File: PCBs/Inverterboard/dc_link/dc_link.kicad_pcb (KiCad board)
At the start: 2 copper layers, 200 x 100.3 mm, 78 parts, among them J2 Conn_02x02_Odd_Even, J3 Conn_02x02_Odd_Even, J4 Conn_02x02_Odd_Even, J5 Conn_02x04_Odd_Even

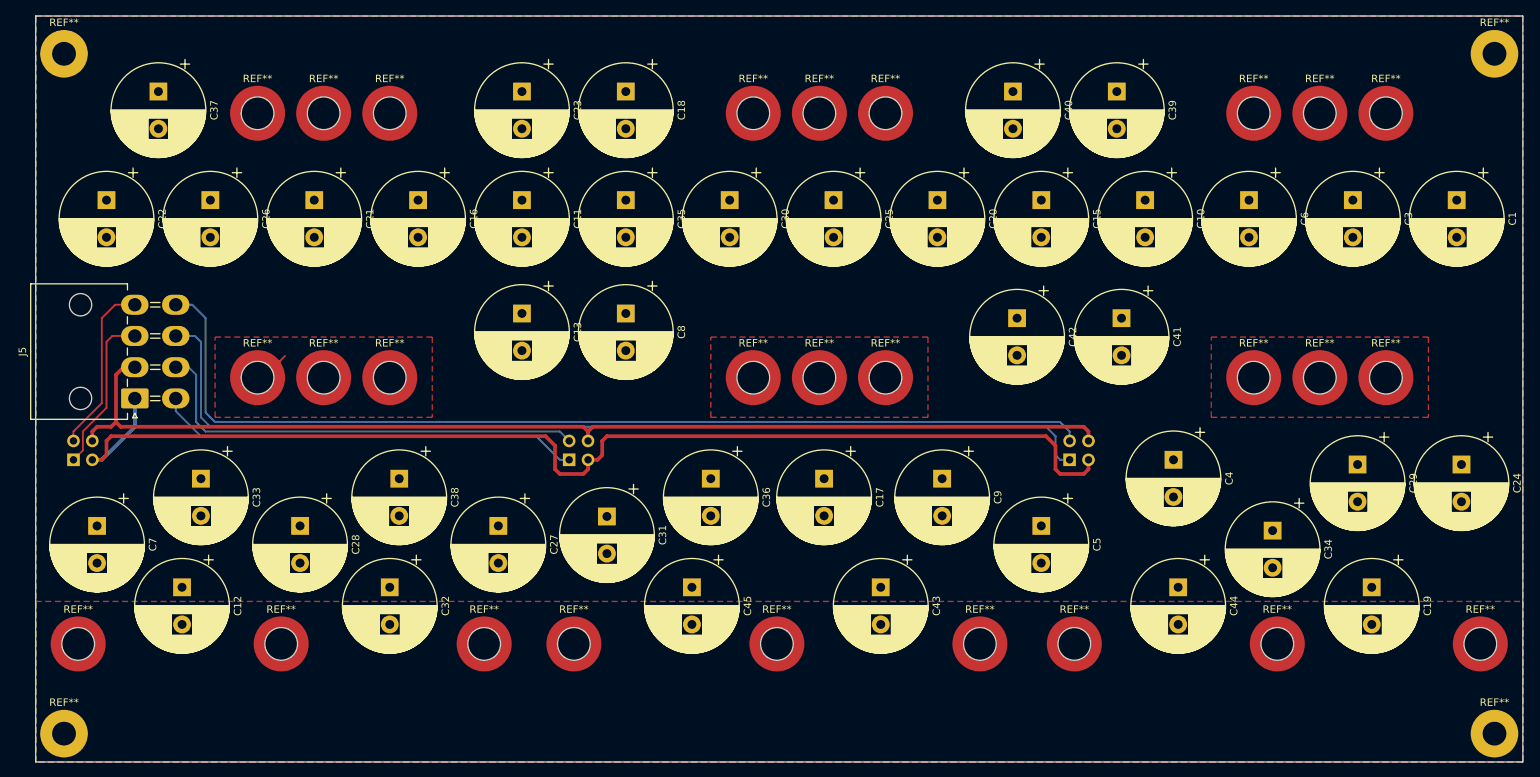
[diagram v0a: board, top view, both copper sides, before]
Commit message: Last fixes after PCB review
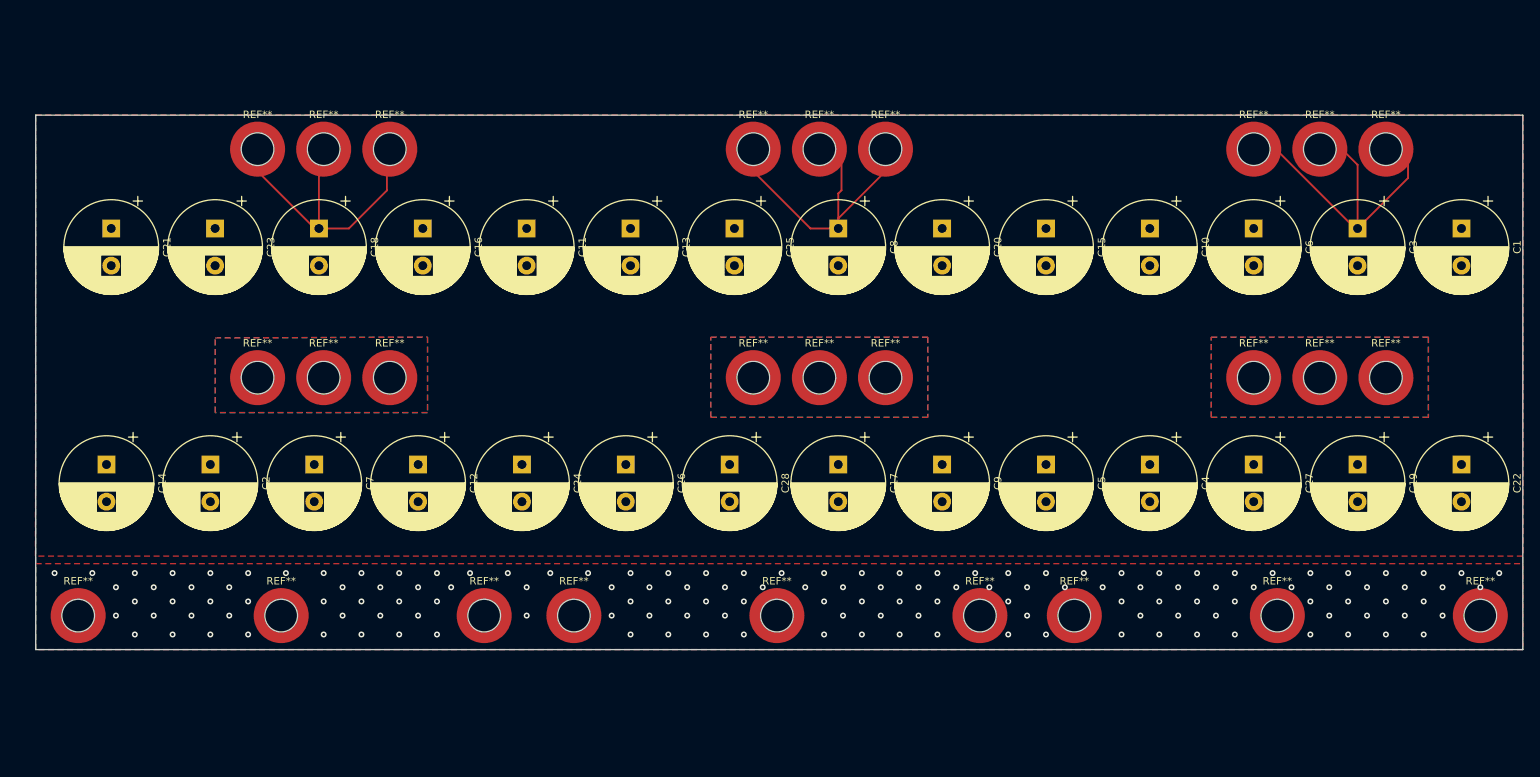
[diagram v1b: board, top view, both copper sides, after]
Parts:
- removed the C21 at (76.8, 62.9)
- removed the C23 at (104.8, 48.3)
- removed the C25 at (146.7, 62.9)
- removed the C27 at (101.6, 106.7)
- removed the C28 at (74.9, 106.7)
- removed C29, C31, C33, C35, C37, C38, C39, C40, C43, C44, C45: CP, Capacitor_THT:CP_Radial_D12.5mm_P5.00mm
- removed J2, J3, J4: Conn_02x02_Odd_Even, Connector_PinSocket_2.54mm:PinSocket_2x02_P2.54mm_Vertical
- removed J5: Conn_02x04_Odd_Even, Connector_Molex:Molex_Mini-Fit_Jr_5569-08A2_2x04_P4.20mm_Horizontal
- removed the REF** at (69.2, 51.2)
- removed the REF** at (45.1, 122.6)
- removed the REF** at (72.4, 122.6)
- removed the REF** at (78.1, 51.2)
- removed the REF** at (99.7, 122.6)
- removed the REF** at (111.8, 122.6)
- removed the REF** at (139.1, 122.6)
- removed the REF** at (166.4, 122.6)
- removed the REF** at (179.1, 122.6)
- removed the REF** at (206.4, 122.6)
- removed the REF** at (233.7, 122.6)
- removed the REF** at (43.2, 43.2)
- removed the REF** at (235.6, 43.2)
- removed the REF** at (235.6, 134.6)
- removed the REF** at (87.0, 51.2)
- removed the REF** at (43.2, 134.6)
- removed the REF** at (221.0, 51.2)
- removed the REF** at (135.9, 51.2)
- removed the REF** at (144.8, 51.2)
- removed the REF** at (153.7, 51.2)
- removed the REF** at (203.2, 51.2)
- removed the REF** at (212.1, 51.2)
- added C24: CP, Capacitor_THT:CP_Radial_D12.5mm_P5.00mm, F.Cu at (104.8, 98.4)
- added REF**: Mounting_Wuerth_WA-SMSR-M3_H2.6mm_ReverseMount_9775026360, Mounting_Wuerth:Mounting_Wuerth_WA-SMSR-M3_H2.6mm_ReverseMount_9775026360, F.Cu at (233.7, 118.7)
- added REF**: Mounting_Wuerth_WA-SMSR-M3_H2.6mm_ReverseMount_9775026360, Mounting_Wuerth:Mounting_Wuerth_WA-SMSR-M3_H2.6mm_ReverseMount_9775026360, F.Cu at (212.1, 56.0)
- added REF**: Mounting_Wuerth_WA-SMSR-M3_H2.6mm_ReverseMount_9775026360, Mounting_Wuerth:Mounting_Wuerth_WA-SMSR-M3_H2.6mm_ReverseMount_9775026360, F.Cu at (203.2, 56.0)
- added REF**: Mounting_Wuerth_WA-SMSR-M3_H2.6mm_ReverseMount_9775026360, Mounting_Wuerth:Mounting_Wuerth_WA-SMSR-M3_H2.6mm_ReverseMount_9775026360, F.Cu at (153.7, 56.0)
- added REF**: Mounting_Wuerth_WA-SMSR-M3_H2.6mm_ReverseMount_9775026360, Mounting_Wuerth:Mounting_Wuerth_WA-SMSR-M3_H2.6mm_ReverseMount_9775026360, F.Cu at (144.8, 56.0)
- added REF**: Mounting_Wuerth_WA-SMSR-M3_H2.6mm_ReverseMount_9775026360, Mounting_Wuerth:Mounting_Wuerth_WA-SMSR-M3_H2.6mm_ReverseMount_9775026360, F.Cu at (135.9, 56.0)
- added REF**: Mounting_Wuerth_WA-SMSR-M3_H2.6mm_ReverseMount_9775026360, Mounting_Wuerth:Mounting_Wuerth_WA-SMSR-M3_H2.6mm_ReverseMount_9775026360, F.Cu at (87.0, 56.0)
- added REF**: Mounting_Wuerth_WA-SMSR-M3_H2.6mm_ReverseMount_9775026360, Mounting_Wuerth:Mounting_Wuerth_WA-SMSR-M3_H2.6mm_ReverseMount_9775026360, F.Cu at (78.1, 56.0)
- added REF**: Mounting_Wuerth_WA-SMSR-M3_H2.6mm_ReverseMount_9775026360, Mounting_Wuerth:Mounting_Wuerth_WA-SMSR-M3_H2.6mm_ReverseMount_9775026360, F.Cu at (206.4, 118.7)
- added REF**: Mounting_Wuerth_WA-SMSR-M3_H2.6mm_ReverseMount_9775026360, Mounting_Wuerth:Mounting_Wuerth_WA-SMSR-M3_H2.6mm_ReverseMount_9775026360, F.Cu at (45.1, 118.7)
- added REF**: Mounting_Wuerth_WA-SMSR-M3_H2.6mm_ReverseMount_9775026360, Mounting_Wuerth:Mounting_Wuerth_WA-SMSR-M3_H2.6mm_ReverseMount_9775026360, F.Cu at (69.2, 56.0)
- added REF**: Mounting_Wuerth_WA-SMSR-M3_H2.6mm_ReverseMount_9775026360, Mounting_Wuerth:Mounting_Wuerth_WA-SMSR-M3_H2.6mm_ReverseMount_9775026360, F.Cu at (179.1, 118.7)
- added REF**: Mounting_Wuerth_WA-SMSR-M3_H2.6mm_ReverseMount_9775026360, Mounting_Wuerth:Mounting_Wuerth_WA-SMSR-M3_H2.6mm_ReverseMount_9775026360, F.Cu at (166.4, 118.7)
- added REF**: Mounting_Wuerth_WA-SMSR-M3_H2.6mm_ReverseMount_9775026360, Mounting_Wuerth:Mounting_Wuerth_WA-SMSR-M3_H2.6mm_ReverseMount_9775026360, F.Cu at (139.1, 118.7)
- added REF**: Mounting_Wuerth_WA-SMSR-M3_H2.6mm_ReverseMount_9775026360, Mounting_Wuerth:Mounting_Wuerth_WA-SMSR-M3_H2.6mm_ReverseMount_9775026360, F.Cu at (111.8, 118.7)
- added REF**: Mounting_Wuerth_WA-SMSR-M3_H2.6mm_ReverseMount_9775026360, Mounting_Wuerth:Mounting_Wuerth_WA-SMSR-M3_H2.6mm_ReverseMount_9775026360, F.Cu at (99.7, 118.7)
- added REF**: Mounting_Wuerth_WA-SMSR-M3_H2.6mm_ReverseMount_9775026360, Mounting_Wuerth:Mounting_Wuerth_WA-SMSR-M3_H2.6mm_ReverseMount_9775026360, F.Cu at (72.4, 118.7)
- added REF**: Mounting_Wuerth_WA-SMSR-M3_H2.6mm_ReverseMount_9775026360, Mounting_Wuerth:Mounting_Wuerth_WA-SMSR-M3_H2.6mm_ReverseMount_9775026360, F.Cu at (221.0, 56.0)
- moved C14 137.9 mm to (48.9, 98.4)
- moved C2 110.3 mm to (62.9, 98.4)
- moved C18 45.2 mm to (77.5, 66.7)
- moved C12 35.8 mm to (90.8, 98.4)
- moved C26 35.8 mm to (118.7, 98.4)
- moved C8 30.8 mm to (147.3, 66.7)
- moved C7 30.4 mm to (76.8, 98.4)
- moved C13 18.5 mm to (119.4, 66.7)
- moved C19 16.6 mm to (217.2, 98.4)
- moved C27 9.25 mm to (203.2, 98.4)
- moved C5 8.28 mm to (175.3, 98.4)
- moved C21 3.86 mm to (49.5, 66.7)
- moved C23 3.86 mm to (63.5, 66.7)
- moved C1 3.86 mm to (231.1, 66.7)
- moved C10 3.86 mm to (189.2, 66.7)
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- renumbered C41 to C14, C42 to C2, C22 to C21, C24 to C22, C26 to C23, C30 to C25, C32 to C26, C34 to C27, C36 to C28
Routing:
- net +12V: track 161.2 -> 0.00 mm
- net +5V: track 148.7 -> 0.00 mm
- net Enable_C: track 136.0 -> 0.00 mm
- net PWM_C: track 134.6 -> 0.00 mm
- net +BATT: track 0.00 -> 109.6 mm
- net Enable_B: track 60.7 -> 0.00 mm
- net PWM_B: track 57.3 -> 0.00 mm
- net Enable_A: track 23.3 -> 0.00 mm
- net PWM_A: track 21.8 -> 0.00 mm
- net PHASE_A: track 3.22 -> 0.00 mm
- net GND: vias 0 -> 146
- added copper zone on B.Cu, net PHASE_A
- added copper zone on B.Cu, net PHASE_B
- added copper zone on B.Cu, net PHASE_C
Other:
- board size 200 x 100.3 mm -> 200 x 71.9 mm
